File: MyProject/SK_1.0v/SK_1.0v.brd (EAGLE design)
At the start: 50 x 50 mm, 37 parts, among them CN2 B2B-ZR, CN4 MICRO-USB-SHIELD-ZX62R-B-5P, IC1 ATMEGA32U4-AU, IC2 MCP73831, IC3 LM2735

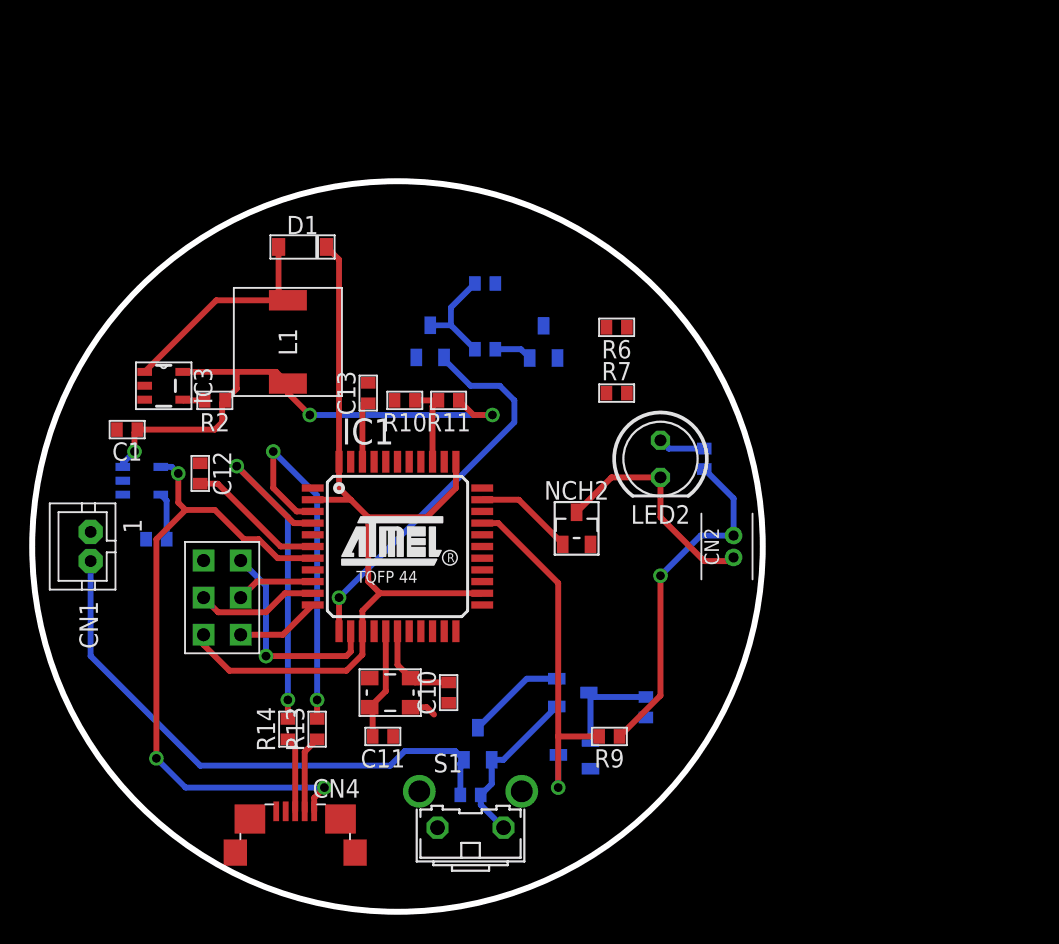
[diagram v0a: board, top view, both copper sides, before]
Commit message: hisashiburi
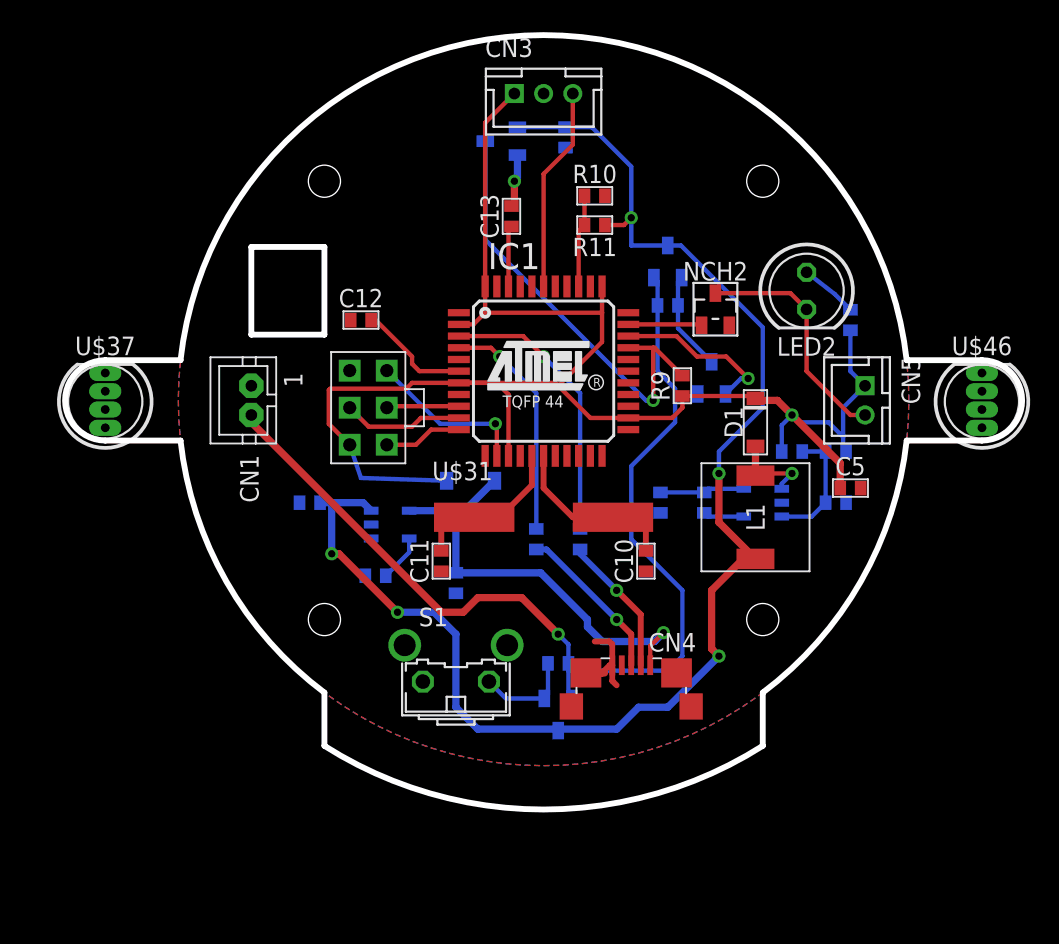
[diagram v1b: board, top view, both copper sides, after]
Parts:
- removed CN2: B2B-ZR, jst:B2B-ZR
- removed PCH3: CHIP_FET_P, 06_FET:SOT23
- removed R4, R6, R7: (no value), 01_R:1608
- added C5: 22uF, 02_C:1608
- added C6: 1nF, 02_C:1608
- added C7, C8: 4.7uF, 02_C:1608
- added CN3: (no value), jst-ph:B3B-PH-K-S
- added CN5: (no value), jst-ph:B2B-PH-K-S
- added D2: SOD-123, 15_DIODE:SOD_123
- added R15: 100K, 01_R:1608
- added R16: 30K, 01_R:1608
- added U$31: CSM-7X-DU, 09_2_CRYSTAL:CSM-7X-DU
- added U$37: NEO5MM, 10_LED:NEO5MM
- C1: value (none) -> 22uF
- L1: value D63 -> 22uH
- R1: value (none) -> 2K
- R2: value (none) -> 100K
- R8, R9: value (none) -> 10K
- U$46: value FA-238 -> NEO5MM; device 09_2_CRYSTAL:FA-238 -> 10_LED:NEO5MM
- moved U$46 45.2 mm to (65.0, 35.0), turned to 0 degrees
- moved NCH3 42.3 mm to (32.1, 52.7)
- moved IC3 41.8 mm to (50.0, 28.0), flipped to the bottom
- moved R8 39.4 mm to (36.5, 53.0)
- moved C1 36.8 mm to (43.0, 28.0), flipped to the bottom, turned to 270 degrees
- moved R2 34.2 mm to (46.0, 28.0), flipped to the bottom, turned to 90 degrees
- moved L1 34.2 mm to (49.5, 27.0)
- moved D1 33.2 mm to (49.5, 33.5), turned to 90 degrees
- moved CN4 25.1 mm to (41.0, 14.0)
- moved R9 24.5 mm to (44.5, 36.0), turned to 270 degrees
- moved R13 22.2 mm to (37.5, 25.5), flipped to the bottom
- moved R14 21.4 mm to (34.5, 25.5), flipped to the bottom
- moved NCH1 19.4 mm to (46.5, 36.5)
- moved R10 19.1 mm to (38.5, 49.0), turned to 180 degrees
- moved NCH2 17.8 mm to (46.8, 41.2)
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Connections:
- net N$15 renamed D9
- net N$16 renamed D8
- removed net N$17: IC1.31
- removed net N$5: NCH3.1, PCH3.3, R8.2
- new net A1: IC1.37
- new net A2: IC1.38
- new net A3: CN3.3, IC1.39
- new net A4: IC1.40
- new net A5: IC1.41
- new net D0: IC1.20
- new net D1: IC1.21
- new net D12: IC1.26
- new net D2: IC1.19
- new net D3: IC1.18
- new net D4: IC1.25
- new net D5: IC1.31, NCH1.1
- new net D6: IC1.27
- new net D7: IC1.1
- new net FB: C6.P$2, IC3.3, R15.2, R16.1
- new net HWB: IC1.33
- new net RXLED: IC1.8
- new net STAT: IC2.1
- new net TXLED: IC1.22
- net +3.7V: now also C7.P$1, NCH3.1, R8.2; no longer PCH3.2, R7.2
- net +5V: now also C5.P$1, C6.P$1, CN3.1, CN5.1, D2.C, IC1.7, R16.2; no longer CN2.1
- net +USB5V: now also C8.P$1, D2.A; no longer IC1.7
- net D11: no longer NCH1.1
- net GND: now also C5.P$2, C7.P$2, C8.P$2, CN3.2, CN4.M1, CN4.M2, CN4.M3, CN4.M4, R15.1; no longer R4.1, R6.1, U$46.2, U$46.4
- net N$1: now also CN5.2; no longer CN2.2
- net N$11: now also U$31.2; no longer U$46.1
- net N$13: now also U$31.1; no longer U$46.3
- net N$6: no longer R4.2
- net SWSIG: no longer PCH3.1, R6.2, R7.1
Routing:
- net +3.7V: track 45.1 -> 106.4 mm, vias 3 -> 5
- net V2: track 40.9 -> 70.5 mm, vias 0 -> 1
- net +5V: track 84.6 -> 111.9 mm
- net D11: track 26.9 -> 0.00 mm, vias 1 -> 0
- net +USB5V: track 46.2 -> 30.5 mm, vias 3 -> 1
- net A3: track 0.00 -> 14.0 mm
- net D5: track 0.00 -> 11.4 mm, vias 0 -> 1
- net N$4: track 15.7 -> 5.91 mm, vias 0 -> 1
- net N$14: track 25.6 -> 15.9 mm, vias 2 -> 1
- net FB: track 0.00 -> 8.49 mm
- net GND: track 1.81 -> 10.1 mm, vias 0 -> 1
- net N$5: track 7.22 -> 0.00 mm
- net N$8: track 25.4 -> 19.2 mm, vias 2 -> 1
- net N$11: track 6.30 -> 12.3 mm
- net D+: track 5.13 -> 11.0 mm, vias 0 -> 1
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- added copper zone on layer 1, net N$5
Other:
- board size 50 x 50 mm -> 65.5 x 53 mm
